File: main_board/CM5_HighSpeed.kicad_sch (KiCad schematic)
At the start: 14 parts, among them J1 USB3_A, J10 Conn_01x22_Female, J22 690-019-298-412, U12 RT9742SNGV, U6 AP22653W6

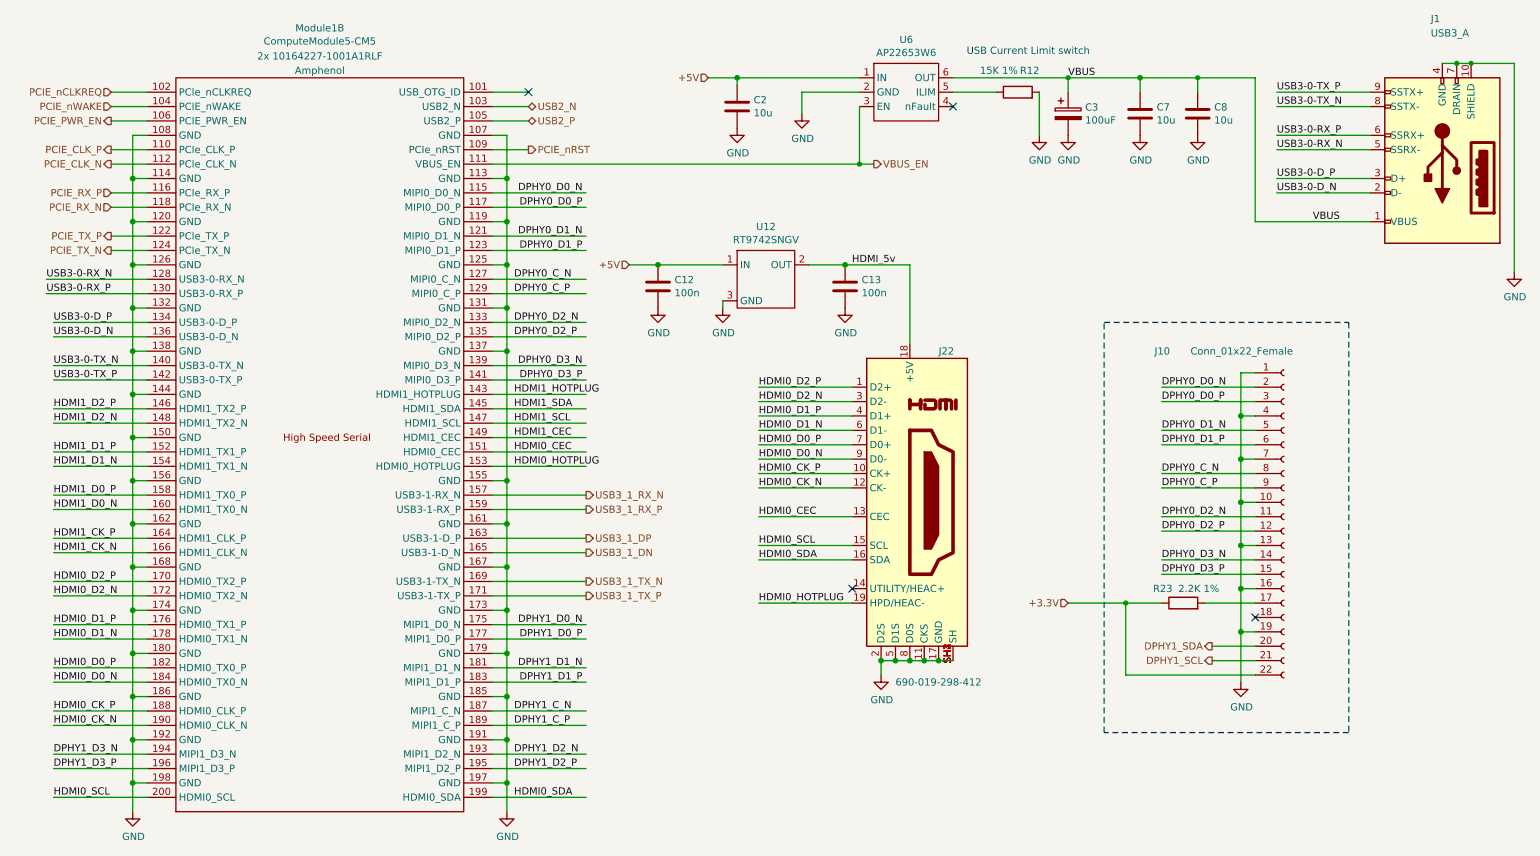
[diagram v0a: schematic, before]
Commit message: Rev 1 draft
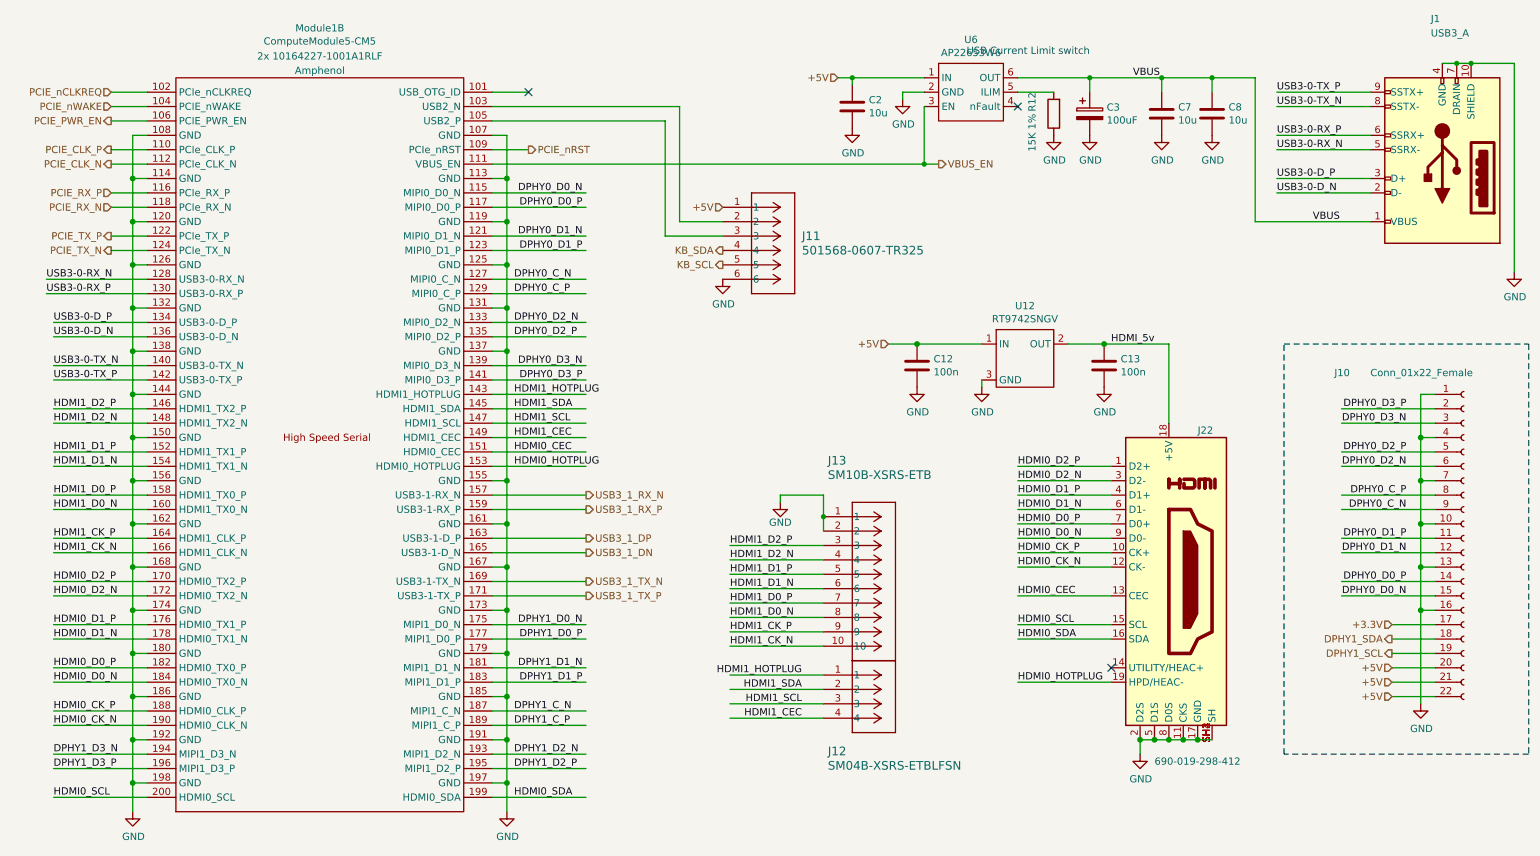
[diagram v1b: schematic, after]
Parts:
- removed R23: 2.2K 1%, Resistor_SMD:R_0805_2012Metric_Pad1.20x1.40mm_HandSolder, symbol Device:R
- added J11: 501568-0607-TR325, CONN_501568-0607-TR325_MOL, symbol 000_Custom:501568-0607-TR325
- added J12: SM04B-XSRS-ETBLFSN, 000_custom:CONN_SM04B-XSRS-ETB_JST, symbol 000_Custom:SM04B-XSRS-ETBLFSN
- added J13: SM10B-XSRS-ETB, 000_custom:CONN_SM10B-XSRS-ETB_JST, symbol 000_Custom:SM10B-XSRS-ETB
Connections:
- net +3.3V: now also J10.17 (Pin_17); no longer J10.22 (Pin_22)
- net +5V: now also J10.20 (Pin_20), J10.21 (Pin_21), J10.22 (Pin_22), J11.1
- net DPHY0_C_N: now also J10.9 (Pin_9); no longer J10.8 (Pin_8)
- net DPHY0_C_P: now also J10.8 (Pin_8); no longer J10.9 (Pin_9)
- net DPHY0_D0_N: now also J10.15 (Pin_15); no longer J10.2 (Pin_2)
- net DPHY0_D0_P: now also J10.14 (Pin_14); no longer J10.3 (Pin_3)
- net DPHY0_D1_N: now also J10.12 (Pin_12); no longer J10.5 (Pin_5)
- net DPHY0_D1_P: now also J10.11 (Pin_11); no longer J10.6 (Pin_6)
- net DPHY0_D2_N: now also J10.6 (Pin_6); no longer J10.11 (Pin_11)
- net DPHY0_D2_P: now also J10.5 (Pin_5); no longer J10.12 (Pin_12)
- net DPHY0_D3_N: now also J10.3 (Pin_3); no longer J10.14 (Pin_14)
- net DPHY0_D3_P: now also J10.2 (Pin_2); no longer J10.15 (Pin_15)
- net DPHY1_SCL: now also J10.19 (Pin_19); no longer J10.21 (Pin_21)
- net DPHY1_SDA: now also J10.18 (Pin_18); no longer J10.20 (Pin_20)
- net GND: now also R12.1, J11.6, J13.1, J13.2; no longer J10.19 (Pin_19), R12.2
- net HDMI1_CEC: now also J12.4
- net HDMI1_CK_N: now also J13.10
- net HDMI1_CK_P: now also J13.9
- net HDMI1_D0_N: now also J13.8
- net HDMI1_D0_P: now also J13.7
- net HDMI1_D1_N: now also J13.6
- net HDMI1_D1_P: now also J13.5
- net HDMI1_D2_N: now also J13.4
- net HDMI1_D2_P: now also J13.3
- net HDMI1_HOTPLUG: now also J12.1
- net HDMI1_SCL: now also J12.3
- net HDMI1_SDA: now also J12.2
- net at U6.5 (ILIM): now also R12.2; no longer R12.1
- net USB2_N: no longer names the net of Module1.103 (USB2_N)
- net USB2_N: now also J11.2
- net USB2_P: no longer names the net of Module1.105 (USB2_P)
- net USB2_P: now also J11.3
- new net KB_SCL: J11.5
- new net KB_SDA: J11.4
- no-connect marks 4 -> 3
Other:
- moved on the sheet: C12, C13, C2, C3, C7, C8, J10, J22, R12, U12, U6
